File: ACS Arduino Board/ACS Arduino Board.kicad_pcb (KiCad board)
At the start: 2 copper layers, 16 parts, among them J1 TBLH10V-350-08BK, J2 TBLH10V-350-02BK, J3 TBLH10V-350-08BK, J4 TBLH10V-350-02BK, J5 MTJ-889X1

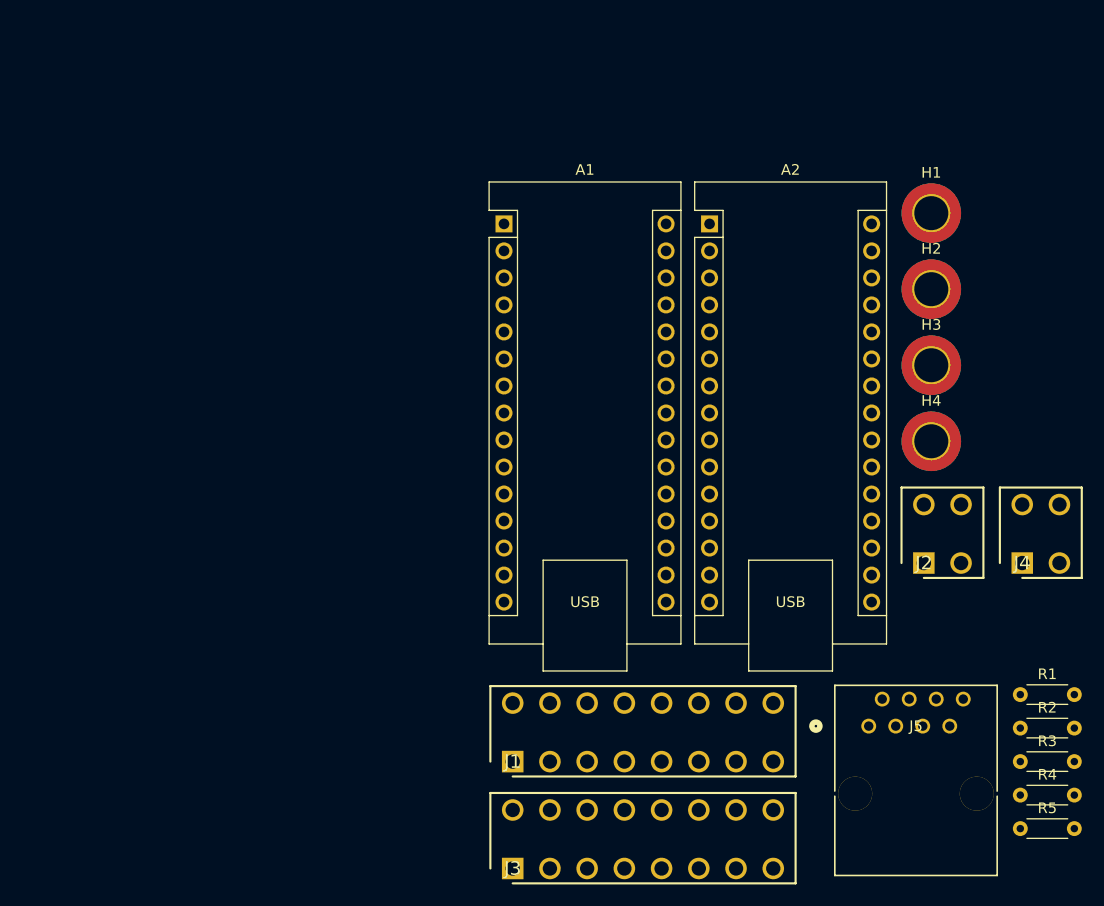
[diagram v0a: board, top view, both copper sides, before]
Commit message: Piss
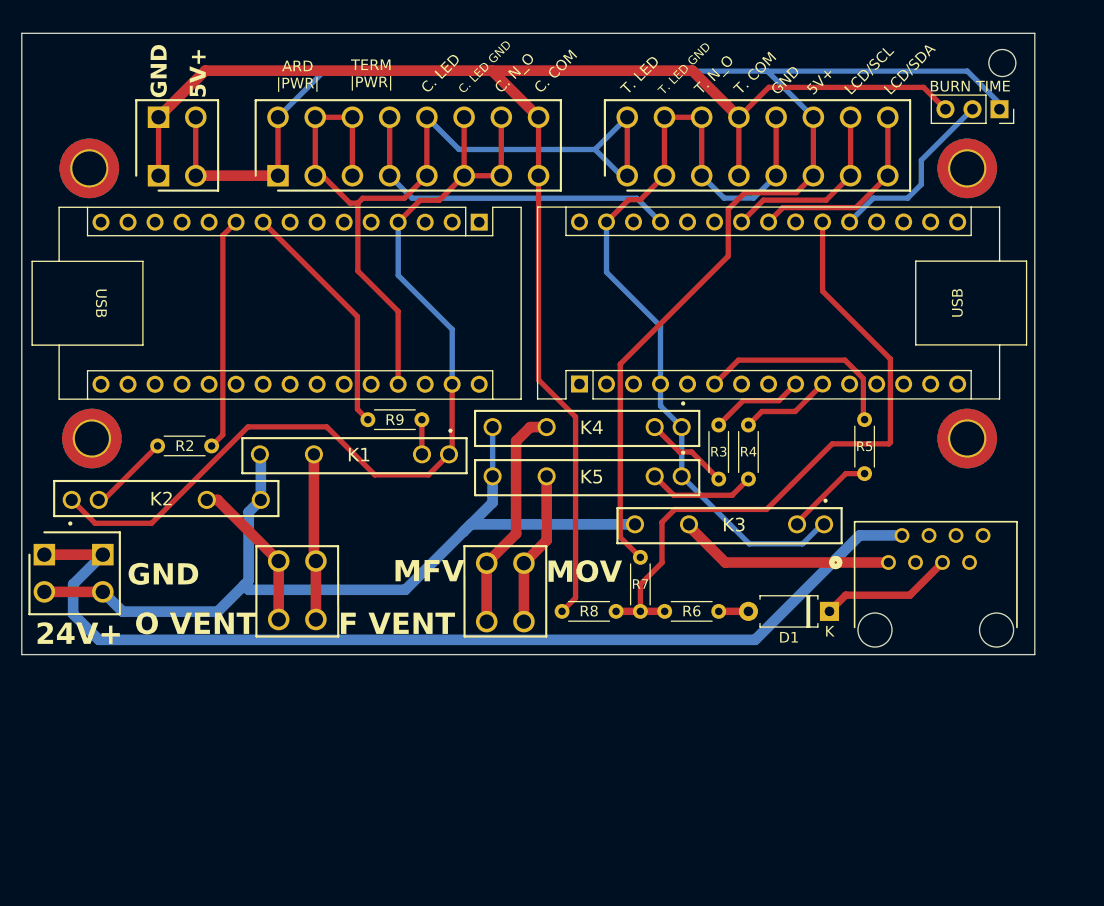
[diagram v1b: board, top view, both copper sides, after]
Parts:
- removed R1: R, Resistor_THT:R_Axial_DIN0204_L3.6mm_D1.6mm_P5.08mm_Horizontal
- added D1: D, Diode_THT:D_A-405_P7.62mm_Horizontal, F.Cu at (101.3, 79.8)
- added J6: TBLH10V-350-08BK, TBLH10V-350-08BK:RHDR16W80P550X350_2X8_2870X850X1420P, F.Cu at (82.3, 38.8)
- added J7: TBLH10V-350-02BK, TBLH10V-350-02BK:RHDR4W80P550X350_2X2_770X850X1420P, F.Cu at (69.1, 80.7)
- added K1: CPC1706Y, RelayCPC:CPC1706Y, F.Cu at (46.1, 66.8)
- added K2: CPC1706Y, RelayCPC:CPC1706Y, F.Cu at (49.5, 67.5)
- added K3: CPC1706Y, RelayCPC:CPC1706Y, F.Cu at (81.4, 73.3)
- added K4: CPC1706Y, RelayCPC:CPC1706Y, F.Cu at (68.0, 64.2)
- added K5: CPC1706Y, RelayCPC:CPC1706Y, F.Cu at (68.0, 68.8)
- added R6: R, Resistor_THT:R_Axial_DIN0204_L3.6mm_D1.6mm_P5.08mm_Horizontal, F.Cu at (90.9, 79.8)
- added R7: R, Resistor_THT:R_Axial_DIN0204_L3.6mm_D1.6mm_P5.08mm_Horizontal, F.Cu at (83.6, 79.8)
- added R8: R, Resistor_THT:R_Axial_DIN0204_L3.6mm_D1.6mm_P5.08mm_Horizontal, F.Cu at (76.2, 79.8)
- added R9: R, Resistor_THT:R_Axial_DIN0204_L3.6mm_D1.6mm_P5.08mm_Horizontal, F.Cu at (63.0, 61.7)
- added RV1: R_Potentiometer, Connector_PinSocket_2.54mm:PinSocket_1x03_P2.54mm_Vertical, F.Cu at (117.3, 32.5)
- J3: value TBLH10V-350-08BK -> TBLH10V-350-02BK; footprint TBLH10V-350-08BK:RHDR16W80P550X350_2X8_2870X850X1420P -> TBLH10V-350-02BK:RHDR4W80P550X350_2X2_770X850X1420P
- moved J4 92.0 mm to (27.5, 74.4), turned to -90 degrees
- moved R2 85.3 mm to (38.2, 64.2)
- moved J2 80.7 mm to (38.3, 38.8)
- moved H1 79.3 mm to (31.8, 38.1)
- moved H4 78.9 mm to (32.0, 63.5)
- moved J1 59.3 mm to (49.5, 38.8)
- moved R4 39.2 mm to (93.7, 67.3), turned to 90 degrees
- moved R3 38.9 mm to (90.9, 67.3), turned to 90 degrees
- moved R5 36.4 mm to (104.6, 66.8), turned to 90 degrees
- moved J3 34.3 mm to (53.1, 75.0), turned to 180 degrees
- moved A2 19.4 mm to (77.8, 58.4), turned to 90 degrees
- moved J5 15.5 mm to (106.9, 75.2)
- moved H2 11.9 mm to (114.3, 38.1)
- moved H3 7.67 mm to (114.3, 63.5)
- moved A1 2.34 mm to (68.4, 43.2), turned to -90 degrees
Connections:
- net OxVent Out renamed Ox Vent Out
- A1 pad 27: Cycle Power -> Arduino Power
- A1 pad 29: GND -> Cycle GND
- A1 pad 4: GND -> Cycle GND
- A2 pad 29: GND -> Terminal GND
- A2 pad 4: GND -> Terminal GND
- H1 pad 1: GND -> unconnected-(H1-Pad1)
- H2 pad 1: GND -> unconnected-(H2-Pad1)
- H3 pad 1: GND -> unconnected-(H3-Pad1)
- H4 pad 1: GND -> unconnected-(H4-Pad1)
- J1 pad 10: Cycle Power -> Arduino Power
- J1 pad 11: Arm Key -> Cycle GND
- J1 pad 12: Arm Key -> Cycle GND
- J1 pad 13: Arm Key -> Cycle GND
- J1 pad 14: Arm Key -> Cycle GND
- J1 pad 15: Terminal Power -> 5V GND
- J1 pad 16: Terminal Power -> 5V GND
- J1 pad 7: Arduino Power -> Terminal Power
- J1 pad 8: Arduino Power -> Terminal Power
- J1 pad 9: Cycle Power -> Arduino Power
- J2 pad 1: GND -> 5V GND
- J2 pad 2: GND -> 5V GND
- J4 pad 1: GND -> 24V GND
- J4 pad 2: GND -> 24V GND
- J5 pad 1: unconnected-(J5-Pad1) -> Ignitor
- J5 pad 2: unconnected-(J5-Pad2) -> 24V GND
- J5 pad 5: unconnected-(J5-Pad5) -> Net-(D1-K)
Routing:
- net +5V: track 0.00 -> 149.3 mm
- net 5V GND: track 0.00 -> 145.3 mm
- net 24V GND: track 0.00 -> 95.3 mm
- net Cycle GND: track 0.00 -> 89.4 mm
- net +24V: track 0.00 -> 83.8 mm
- net Arduino Power: track 0.00 -> 82.1 mm
- net Terminal GND: track 0.00 -> 79.4 mm
- net Break Wire: track 0.00 -> 61.7 mm
- net Terminal Power: track 0.00 -> 32.8 mm
- net Net-(A1-D6): track 0.00 -> 22.7 mm
- net Net-(A1-D7): track 0.00 -> 22.0 mm
- net Main Fuel Out: track 0.00 -> 21.5 mm
- net Ignitor: track 0.00 -> 20.4 mm
- net Net-(A2-D3): track 0.00 -> 19.5 mm
- net LCD/SDA: track 0.00 -> 18.5 mm
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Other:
- board outline added: 95.2 x 58.4 mm
- board text added: "24V+"
- board text added: "5V+"
- board text added: "ARD |PWR|"
- board text added: "BURN TIME"
- board text added: "C. COM"
- board text added: "C. LED"
- board text added: "C. LED GND"
- board text added: "C. N_O"
- board text added: "F VENT"
- board text added: "GND"
- board text added: "LCD/SCL"
- board text added: "LCD/SDA"
- board text added: "MFV"
- board text added: "MOV"
- board text added: "O VENT"
- board text added: "T. COM"
- board text added: "T. LED"
- board text added: "T. LED GND"
- board text added: "T. N_O"
- board text added: "TERM |PWR|"
